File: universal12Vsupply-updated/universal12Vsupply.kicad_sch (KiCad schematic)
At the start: 62 parts, among them J1 Screw_Terminal_01x04, J2 Screw_Terminal_01x02, SW1 TestPoint, U1 LM5175PWP

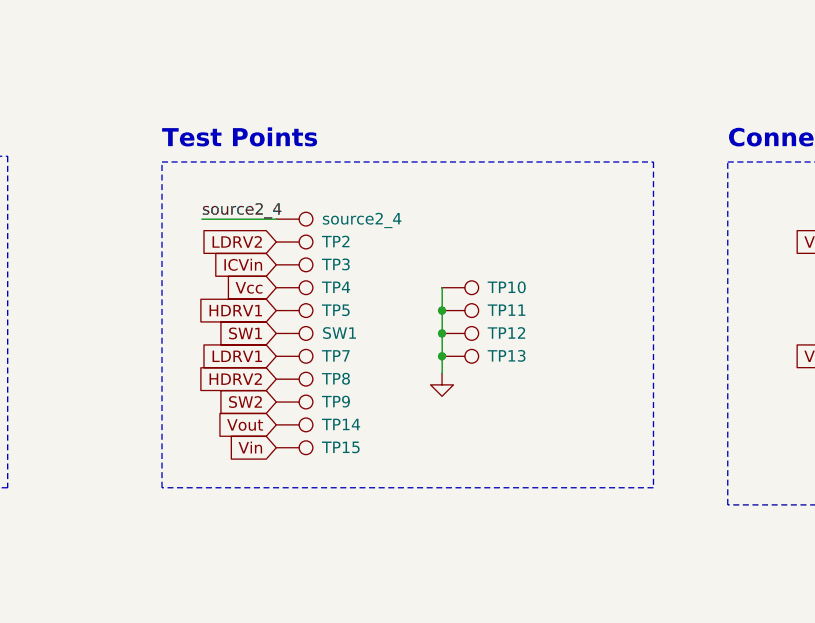
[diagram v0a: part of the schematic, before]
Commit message: design clean up
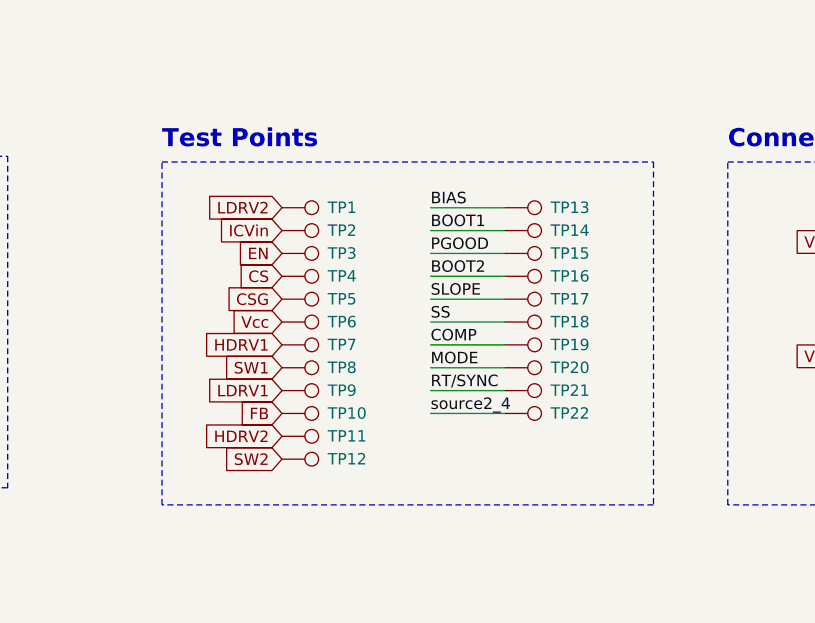
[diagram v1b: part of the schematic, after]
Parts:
- removed TP11, TP12: TestPoint, TestPoint:TestPoint_THTPad_2.5x2.5mm_Drill1.2mm, symbol Connector:TestPoint
- added TP16, TP17, TP18, TP19, TP20, TP21, TP3, TP4, TP5: TestPoint, symbol Connector:TestPoint
- TP1: renamed from TP2; footprint TestPoint:TestPoint_THTPad_2.5x2.5mm_Drill1.2mm -> (none)
- TP10, TP13, TP14, TP15: footprint TestPoint:TestPoint_THTPad_2.5x2.5mm_Drill1.2mm -> (none)
- TP11: renamed from TP8; footprint TestPoint:TestPoint_THTPad_2.5x2.5mm_Drill1.2mm -> (none)
- TP12: renamed from TP9; footprint TestPoint:TestPoint_THTPad_2.5x2.5mm_Drill1.2mm -> (none)
- TP2: renamed from TP3; footprint TestPoint:TestPoint_THTPad_2.5x2.5mm_Drill1.2mm -> (none)
- TP22: renamed from source2_4; footprint TestPoint:TestPoint_THTPad_2.5x2.5mm_Drill1.2mm -> (none)
- TP6: renamed from TP4; footprint TestPoint:TestPoint_THTPad_2.5x2.5mm_Drill1.2mm -> (none)
- TP7: renamed from TP5; footprint TestPoint:TestPoint_THTPad_2.5x2.5mm_Drill1.2mm -> (none)
- TP8: renamed from SW1; footprint TestPoint:TestPoint_THTPad_2.5x2.5mm_Drill1.2mm -> (none)
- TP9: renamed from TP7; footprint TestPoint:TestPoint_THTPad_2.5x2.5mm_Drill1.2mm -> (none)
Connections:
- net BIAS: now also TP13.1
- net BOOT1: now also TP14.1
- net BOOT2: now also TP16.1
- net COMP: now also TP19.1
- net CS: now also TP4.1
- net CSG: now also TP5.1
- net EN: now also TP3.1
- net FB: now also TP10.1
- net GND: no longer TP10.1, TP13.1
- net MODE: now also TP20.1
- net PGOOD: now also TP15.1
- net RT/SYNC: now also TP21.1
- net SLOPE: now also TP17.1
- net SS: now also TP18.1
- net Vin: no longer TP15.1
- net Vout: no longer TP14.1
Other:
- moved on the sheet: TP1, TP11, TP12, TP2, TP22, TP6, TP7, TP8, TP9
